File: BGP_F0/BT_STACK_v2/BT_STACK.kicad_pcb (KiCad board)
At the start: 2 copper layers, 24 x 26 mm, 20 parts, among them P1 CONN_01X05, P2 CONN_01X02, P3 CONN_01X04, U1 MC33178

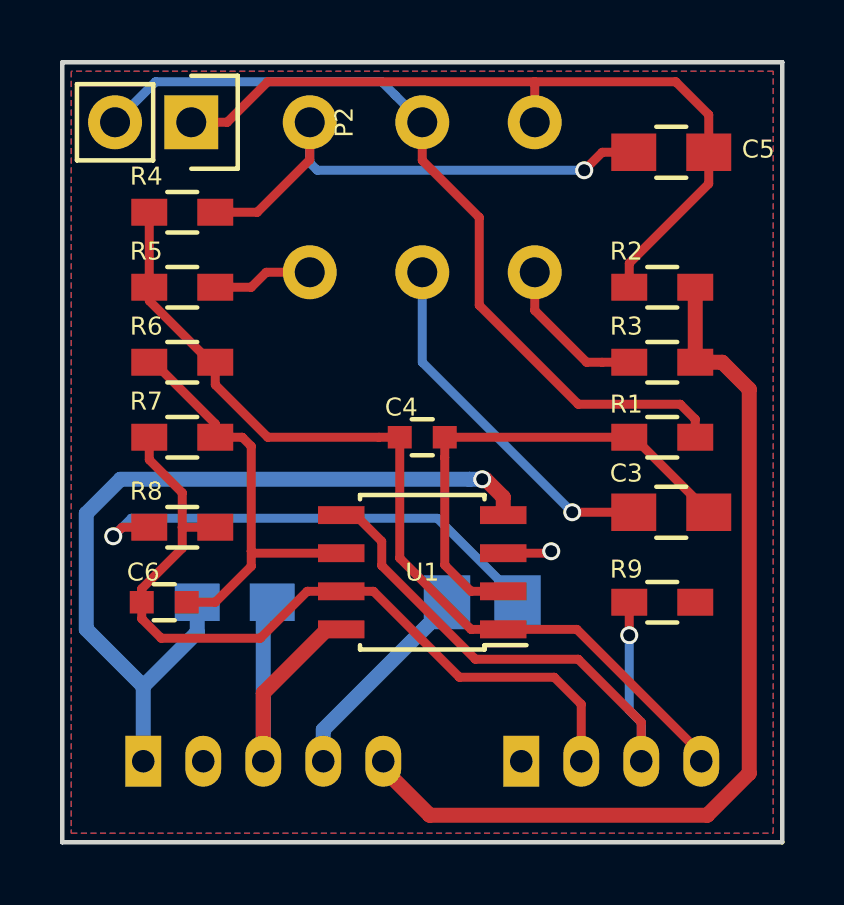
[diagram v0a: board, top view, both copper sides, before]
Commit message: Slight changes
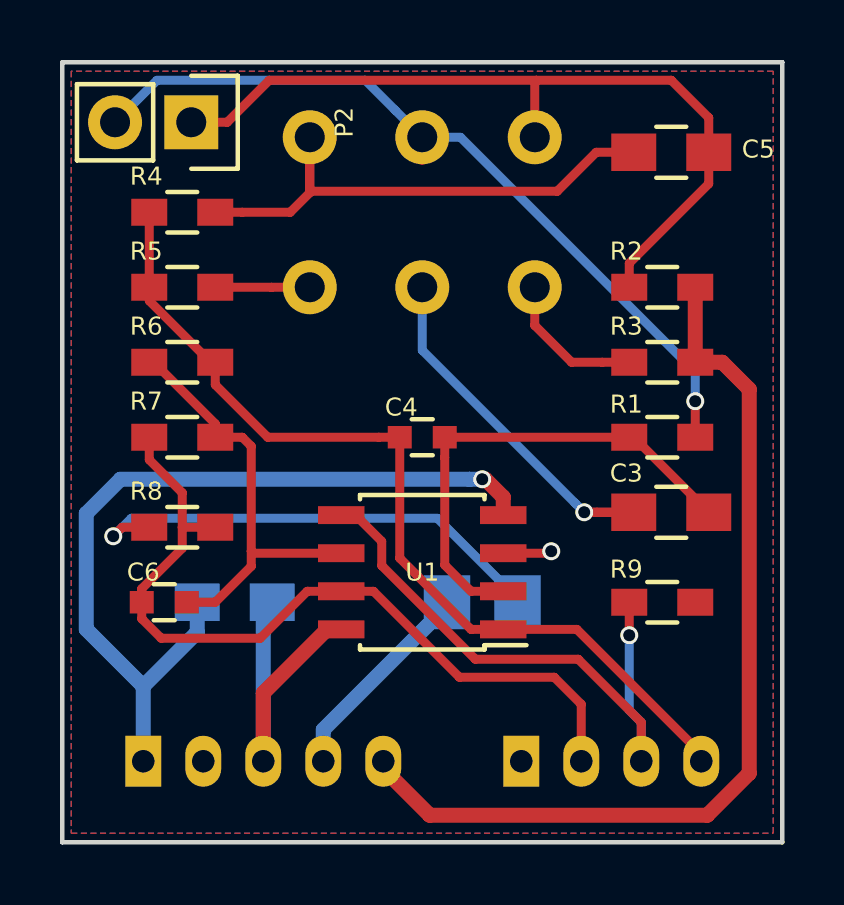
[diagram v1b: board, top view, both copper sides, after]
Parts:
- moved RV1 0.50 mm to (148.2, 71.5)
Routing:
- net /B-: track 17.6 -> 21.0 mm, vias 1 -> 0
- net /T+: track 5.14 -> 6.20 mm
- net /TW: track 12.1 -> 13.0 mm
- net /BW: track 27.6 -> 27.4 mm, vias 0 -> 1
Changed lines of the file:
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@@
     (links 38)
     (no_connects 0)
-    (area 139.924999 68.924999 164.075001 95.075001)
+    (area 139.674999 66.864286 164.085715 95.075001)
     (thickness 1.6)
     (drawings 8)
-    (tracks 142)
+    (tracks 146)
     (zones 0)
     (modules 20)
@@
   )
   (module LIBS:Potentiometer_Alpha_Double_Vertical_Dual_Shaft (layer B.Cu)
-    (at 148.25 71 90)
+    (at 148.25 71.5 90)
     (descr "Potentiometer, vertically mounted, Omeg PC16PU, Omeg PC16PU, Omeg PC16PU, Vishay/Spectrol 248GJ/249GJ Single, Vishay/Spectrol 248GJ/249GJ Single, Vishay/Spectrol 248GJ/249GJ Single, Vishay/Spectrol 248GH/249GH Single, Vishay/Spectrol 148/149 Single, Vishay/Spectrol 148/149 Single, Vishay/Spectrol 148/149 Single, Vishay/Spectrol 148A/149A Single with mounting plates, Vishay/Spectrol 148/149 Double, Vishay/Spectrol 148A/149A Double with mounting plates, Piher PC-16 Single, Piher PC-16 Single, Piher PC-16 Single, Piher PC-16SV Single, Piher PC-16 Double, Piher PC-16 Triple, Piher T16H Single, Piher T16L Single, Piher T16H Double, Alps RK163 Single, Alps RK163 Double, Alps RK097 Single, Alps RK097 Double, http://www.alps.com/prod/info/E/HTML/Potentiometer/RotaryPotentiometers/RK097/RK09712100AV.html")
     (tags "Potentiometer vertical  Omeg PC16PU  Omeg PC16PU  Omeg PC16PU  Vishay/Spectrol 248GJ/249GJ Single  Vishay/Spectrol 248GJ/249GJ Single  Vishay/Spectrol 248GJ/249GJ Single  Vishay/Spectrol 248GH/249GH Single  Vishay/Spectrol 148/149 Single  Vishay/Spectrol 148/149 Single  Vishay/Spectrol 148/149 Single  Vishay/Spectrol 148A/149A Single with mounting plates  Vishay/Spectrol 148/149 Double  Vishay/Spectrol 148A/149A Double with mounting plates  Piher PC-16 Single  Piher PC-16 Single  Piher PC-16 Single  Piher PC-16SV Single  Piher PC-16 Double  Piher PC-16 Triple  Piher T16H Single  Piher T16L Single  Piher T16H Double  Alps RK163 Single  Alps RK163 Double  Alps RK097 Single  Alps RK097 Double Dual Shaft")
-    (fp_text reference RV1 (at -12.3 9.75 180) (layer B.SilkS)
+    (fp_text reference RV1 (at -11.2 9.55 180) (layer B.SilkS)
       (effects (font (size 0.6 0.6) (thickness 0.15)) (justify mirror))
     )
@@
   (segment (start 152.82398 87.12573) (end 148.7 91.24971) (width 0.5) (layer B.Cu) (net 4))
   (segment (start 148.7 91.24971) (end 148.7 92.3) (width 0.5) (layer B.Cu) (net 4))
-  (segment (start 157 84) (end 159.05 84) (width 0.3) (layer F.Cu) (net 5))
-  (segment (start 152 76) (end 152 79) (width 0.3) (layer B.Cu) (net 5))
-  (segment (start 152 79) (end 157 84) (width 0.3) (layer B.Cu) (net 5))
-  (via (at 157 84) (size 0.6) (drill 0.4) (layers F.Cu B.Cu) (net 5))
+  (segment (start 158.95 84.1) (end 158.85 84) (width 0.3) (layer F.Cu) (net 5))
+  (segment (start 157.100001 83.700001) (end 157.4 84) (width 0.3) (layer B.Cu) (net 5))
+  (segment (start 152 78.6) (end 157.100001 83.700001) (width 0.3) (layer B.Cu) (net 5))
+  (segment (start 158.85 84) (end 157.824264 84) (width 0.3) (layer F.Cu) (net 5))
+  (segment (start 152 76.5) (end 152 78.6) (width 0.3) (layer B.Cu) (net 5))
+  (segment (start 157.824264 84) (end 157.4 84) (width 0.3) (layer F.Cu) (net 5))
+  (segment (start 159.05 84) (end 157.4 84) (width 0.3) (layer F.Cu) (net 5))
+  (via (at 157.4 84) (size 0.6) (drill 0.4) (layers F.Cu B.Cu) (net 5))
   (segment (start 154.7 86.635) (end 153.625 86.635) (width 0.3) (layer F.Cu) (net 6))
   (segment (start 153.625 86.635) (end 152.75 85.76) (width 0.3) (layer F.Cu) (net 6))
@@
   (segment (start 145.1 79) (end 144.95 79) (width 0.3) (layer F.Cu) (net 7))
   (segment (start 144.95 79) (end 142.9 76.95) (width 0.3) (layer F.Cu) (net 7))
-  (segment (start 160.449999 69.649999) (end 161.55 70.75) (width 0.3) (layer F.Cu) (net 8))
-  (segment (start 161.55 70.75) (end 161.55 72) (width 0.3) (layer F.Cu) (net 8))
-  (segment (start 155.75 69.649999) (end 160.449999 69.649999) (width 0.3) (layer F.Cu) (net 8))
+  (segment (start 155.75 71.5) (end 155.75 69.65) (width 0.3) (layer F.Cu) (net 8))
+  (segment (start 155.75 69.65) (end 155.8 69.6) (width 0.3) (layer F.Cu) (net 8))
+  (segment (start 146.9 69.6) (end 155.8 69.6) (width 0.3) (layer F.Cu) (net 8))
+  (segment (start 155.8 69.6) (end 160.3 69.6) (width 0.3) (layer F.Cu) (net 8))
   (segment (start 144.3 71) (end 145.5 71) (width 0.3) (layer F.Cu) (net 8))
-  (segment (start 145.5 71) (end 146.850001 69.649999) (width 0.3) (layer F.Cu) (net 8))
-  (segment (start 146.850001 69.649999) (end 155.75 69.649999) (width 0.3) (layer F.Cu) (net 8))
-  (segment (start 155.75 69.649999) (end 155.75 71) (width 0.3) (layer F.Cu) (net 8))
+  (segment (start 145.5 71) (end 146.9 69.6) (width 0.3) (layer F.Cu) (net 8))
+  (segment (start 161.55 70.85) (end 161.55 72) (width 0.3) (layer F.Cu) (net 8))
+  (segment (start 160.3 69.6) (end 161.55 70.85) (width 0.3) (layer F.Cu) (net 8))
   (segment (start 158.9 75.7) (end 161.55 73.05) (width 0.3) (layer F.Cu) (net 8))
   (segment (start 161.55 73.05) (end 161.55 72) (width 0.3) (layer F.Cu) (net 8))
   (segment (start 158.9 76.5) (end 158.9 75.7) (width 0.3) (layer F.Cu) (net 8))
-  (segment (start 161.425 72) (end 161.55 72) (width 0.3) (layer F.Cu) (net 8))
-  (segment (start 145.1 74) (end 146.5 74) (width 0.3) (layer F.Cu) (net 9))
-  (segment (start 146.5 74) (end 148.25 72.25) (width 0.3) (layer F.Cu) (net 9))
+  (segment (start 159.05 72) (end 157.8 72) (width 0.3) (layer F.Cu) (net 9))
+  (segment (start 156.5 73.3) (end 148.25 73.3) (width 0.3) (layer F.Cu) (net 9))
+  (segment (start 157.8 72) (end 156.5 73.3) (width 0.3) (layer F.Cu) (net 9))
+  (segment (start 148.25 73.3) (end 148.25 71.5) (width 0.3) (layer F.Cu) (net 9))
+  (segment (start 148.25 71.5) (end 148.25 73.35) (width 0.3) (layer F.Cu) (net 9))
+  (segment (start 146 74) (end 145.1 74) (width 0.3) (layer F.Cu) (net 9))
+  (segment (start 148.25 73.35) (end 147.6 74) (width 0.3) (layer F.Cu) (net 9))
+  (segment (start 147.6 74) (end 146 74) (width 0.3) (layer F.Cu) (net 9))
   (segment (start 148.25 72.25) (end 148.25 71) (width 0.3) (layer F.Cu) (net 9))
-  (segment (start 157.4 72.6) (end 148.5 72.6) (width 0.3) (layer B.Cu) (net 9))
-  (segment (start 148.5 72.6) (end 148.25 72.35) (width 0.3) (layer B.Cu) (net 9))
   (segment (start 148.25 72.35) (end 148.25 71) (width 0.3) (layer B.Cu) (net 9))
-  (segment (start 159.05 72) (end 158 72) (width 0.3) (layer F.Cu) (net 9))
-  (segment (start 158 72) (end 157.4 72.6) (width 0.3) (layer F.Cu) (net 9))
-  (via (at 157.4 72.6) (size 0.6) (drill 0.4) (layers F.Cu B.Cu) (net 9))
   (segment (start 154.7 85.365) (end 156.235 85.365) (width 0.3) (layer F.Cu) (net 10))
   (segment (start 156.235 85.365) (end 156.3 85.3) (width 0.3) (layer F.Cu) (net 10))
@@
   (segment (start 153.771458 88.9) (end 157.2 88.9) (width 0.3) (layer F.Cu) (net 12))
   (segment (start 159.3 91) (end 159.3 92.3) (width 0.3) (layer F.Cu) (net 12))
-  (segment (start 141.76 71) (end 143.110001 69.649999) (width 0.3) (layer B.Cu) (net 13))
-  (segment (start 151.100001 70.100001) (end 152 71) (width 0.3) (layer B.Cu) (net 13))
-  (segment (start 143.110001 69.649999) (end 150.649999 69.649999) (width 0.3) (layer B.Cu) (net 13))
-  (segment (start 150.649999 69.649999) (end 151.100001 70.100001) (width 0.3) (layer B.Cu) (net 13))
+  (segment (start 161.1 80.3) (end 161.1 81.5) (width 0.3) (layer F.Cu) (net 13))
+  (segment (start 152 71.5) (end 153.272792 71.5) (width 0.3) (layer B.Cu) (net 13))
+  (segment (start 153.272792 71.5) (end 161.1 79.327208) (width 0.3) (layer B.Cu) (net 13))
+  (segment (start 161.1 79.327208) (end 161.1 80.3) (width 0.3) (layer B.Cu) (net 13))
+  (via (at 161.1 80.3) (size 0.6) (drill 0.4) (layers F.Cu B.Cu) (net 13))
+  (segment (start 141.76 71) (end 143.16 69.6) (width 0.3) (layer B.Cu) (net 13))
+  (segment (start 143.16 69.6) (end 150.1 69.6) (width 0.3) (layer B.Cu) (net 13))
+  (segment (start 150.1 69.6) (end 151.100001 70.600001) (width 0.3) (layer B.Cu) (net 13))
+  (segment (start 151.100001 70.600001) (end 152 71.5) (width 0.3) (layer B.Cu) (net 13))
   (segment (start 152 71) (end 152 72.272792) (width 0.3) (layer F.Cu) (net 13))
-  (segment (start 153.9 77.1) (end 157.2 80.4) (width 0.3) (layer F.Cu) (net 13))
-  (segment (start 152 72.272792) (end 153.9 74.172792) (width 0.3) (layer F.Cu) (net 13))
-  (segment (start 153.9 74.172792) (end 153.9 77.1) (width 0.3) (layer F.Cu) (net 13))
-  (segment (start 161.1 80.9) (end 161.1 81.5) (width 0.3) (layer F.Cu) (net 13))
-  (segment (start 157.2 80.4) (end 160.6 80.4) (width 0.3) (layer F.Cu) (net 13))
-  (segment (start 160.6 80.4) (end 161.1 80.9) (width 0.3) (layer F.Cu) (net 13))
-  (segment (start 148.25 76) (end 146.8 76) (width 0.3) (layer F.Cu) (net 14))
-  (segment (start 146.3 76.5) (end 145.1 76.5) (width 0.3) (layer F.Cu) (net 14))
-  (segment (start 146.8 76) (end 146.3 76.5) (width 0.3) (layer F.Cu) (net 14))
+  (segment (start 148.25 76.5) (end 146.977208 76.5) (width 0.3) (layer F.Cu) (net 14))
+  (segment (start 146.977208 76.5) (end 145.1 76.5) (width 0.3) (layer F.Cu) (net 14))
+  (segment (start 155.75 76.5) (end 155.75 77.772792) (width 0.3) (layer F.Cu) (net 15))
+  (segment (start 155.75 77.772792) (end 156.977208 79) (width 0.3) (layer F.Cu) (net 15))
+  (segment (start 156.977208 79) (end 158 79) (width 0.3) (layer F.Cu) (net 15))
+  (segment (start 158 79) (end 158.9 79) (width 0.3) (layer F.Cu) (net 15))
   (segment (start 155.75 76) (end 155.75 77.272792) (width 0.3) (layer F.Cu) (net 15))
-  (segment (start 155.75 77.272792) (end 157.477208 79) (width 0.3) (layer F.Cu) (net 15))
-  (segment (start 157.477208 79) (end 158 79) (width 0.3) (layer F.Cu) (net 15))
-  (segment (start 158 79) (end 158.9 79) (width 0.3) (layer F.Cu) (net 15))
   (segment (start 142.9 79) (end 143.05 79) (width 0.3) (layer F.Cu) (net 16))
   (segment (start 145.1 81.05) (end 145.1 81.5) (width 0.3) (layer F.Cu) (net 16))
